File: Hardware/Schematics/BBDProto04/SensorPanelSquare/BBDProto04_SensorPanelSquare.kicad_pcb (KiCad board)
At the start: 2 copper layers, 223.5 x 238.8 mm, 94 parts, among them P1 CONN_02X08, P1-01 CONN_01X01, P1-02 CONN_01X01, P1-03 CONN_01X01, P1-04 CONN_01X01, P1-05 CONN_01X01, P1-06 CONN_01X01, P1-07 CONN_01X01, P1-08 CONN_01X01, P1-09 CONN_01X01, P1-10 CONN_01X01, P1-11 CONN_01X01, P1-12 CONN_01X01, P1-13 CONN_01X01, P1-14 CONN_01X01, P1-15 CONN_01X01, P1-16 CONN_01X01, P2 CONN_02X08, P2-01 CONN_01X01, P2-02 CONN_01X01, P2-03 CONN_01X01, P2-04 CONN_01X01, P2-05 CONN_01X01, P2-06 CONN_01X01, P2-07 CONN_01X01, P2-08 CONN_01X01, P2-09 CONN_01X01, P2-10 CONN_01X01, P2-11 CONN_01X01, P2-12 CONN_01X01, P2-13 CONN_01X01, P2-14 CONN_01X01, P2-15 CONN_01X01, P2-16 CONN_01X01, P3 CONN_02X08, P3-01 CONN_01X01, P3-02 CONN_01X01, P3-03 CONN_01X01, P3-04 CONN_01X01, P3-05 CONN_01X01, P3-06 CONN_01X01, P3-07 CONN_01X01, P3-08 CONN_01X01, P3-09 CONN_01X01, P3-10 CONN_01X01, P3-11 CONN_01X01, P3-12 CONN_01X01, P3-13 CONN_01X01, P3-14 CONN_01X01, P3-15 CONN_01X01, P3-16 CONN_01X01, P4 CONN_02X08, P4-01 CONN_01X01, P4-02 CONN_01X01, P4-03 CONN_01X01, P4-04 CONN_01X01, P4-05 CONN_01X01, P4-06 CONN_01X01, P4-07 CONN_01X01, P4-08 CONN_01X01, P4-09 CONN_01X01, P4-10 CONN_01X01, P4-11 CONN_01X01, P4-12 CONN_01X01, P4-13 CONN_01X01, P4-14 CONN_01X01, P4-15 CONN_01X01, P4-16 CONN_01X01

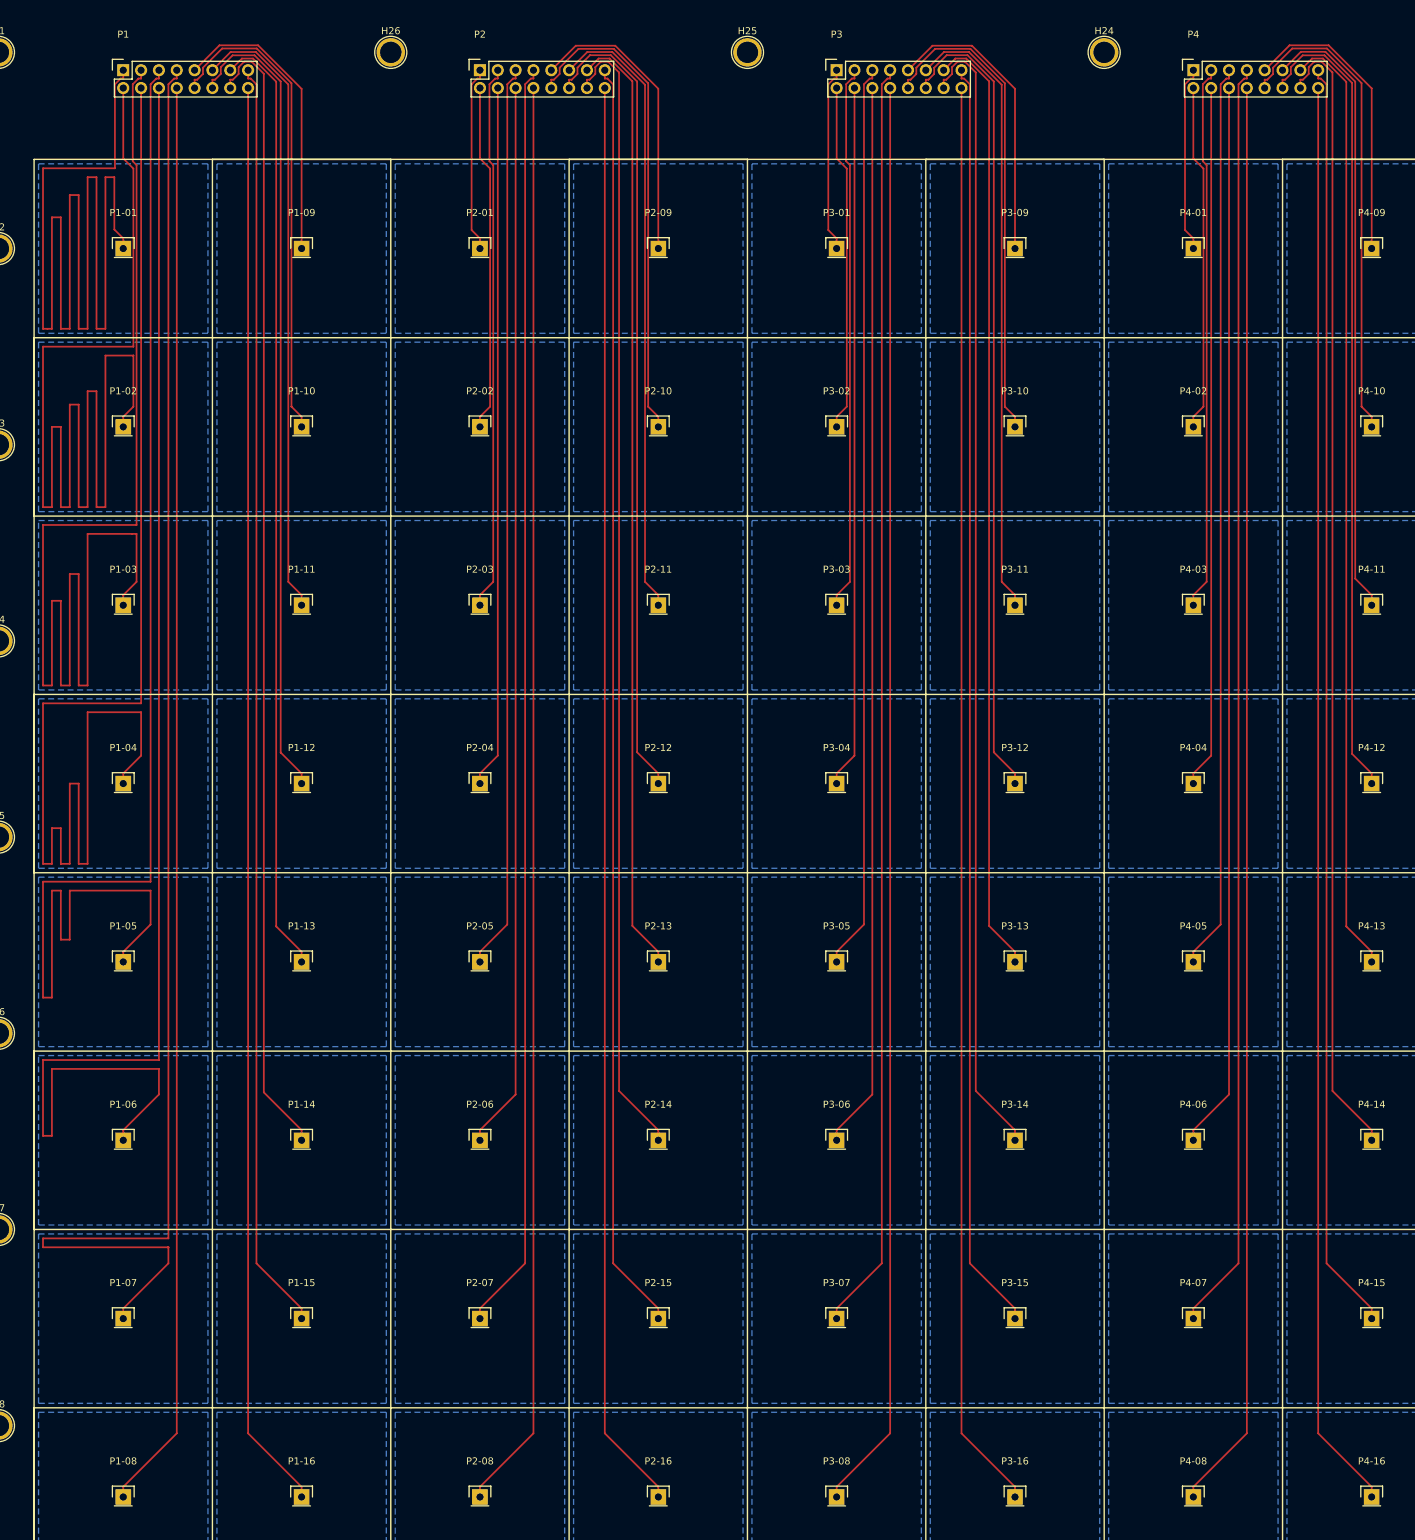
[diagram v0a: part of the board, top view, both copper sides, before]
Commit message: Proto #4 - Rev A
Proto #4 - Rev A
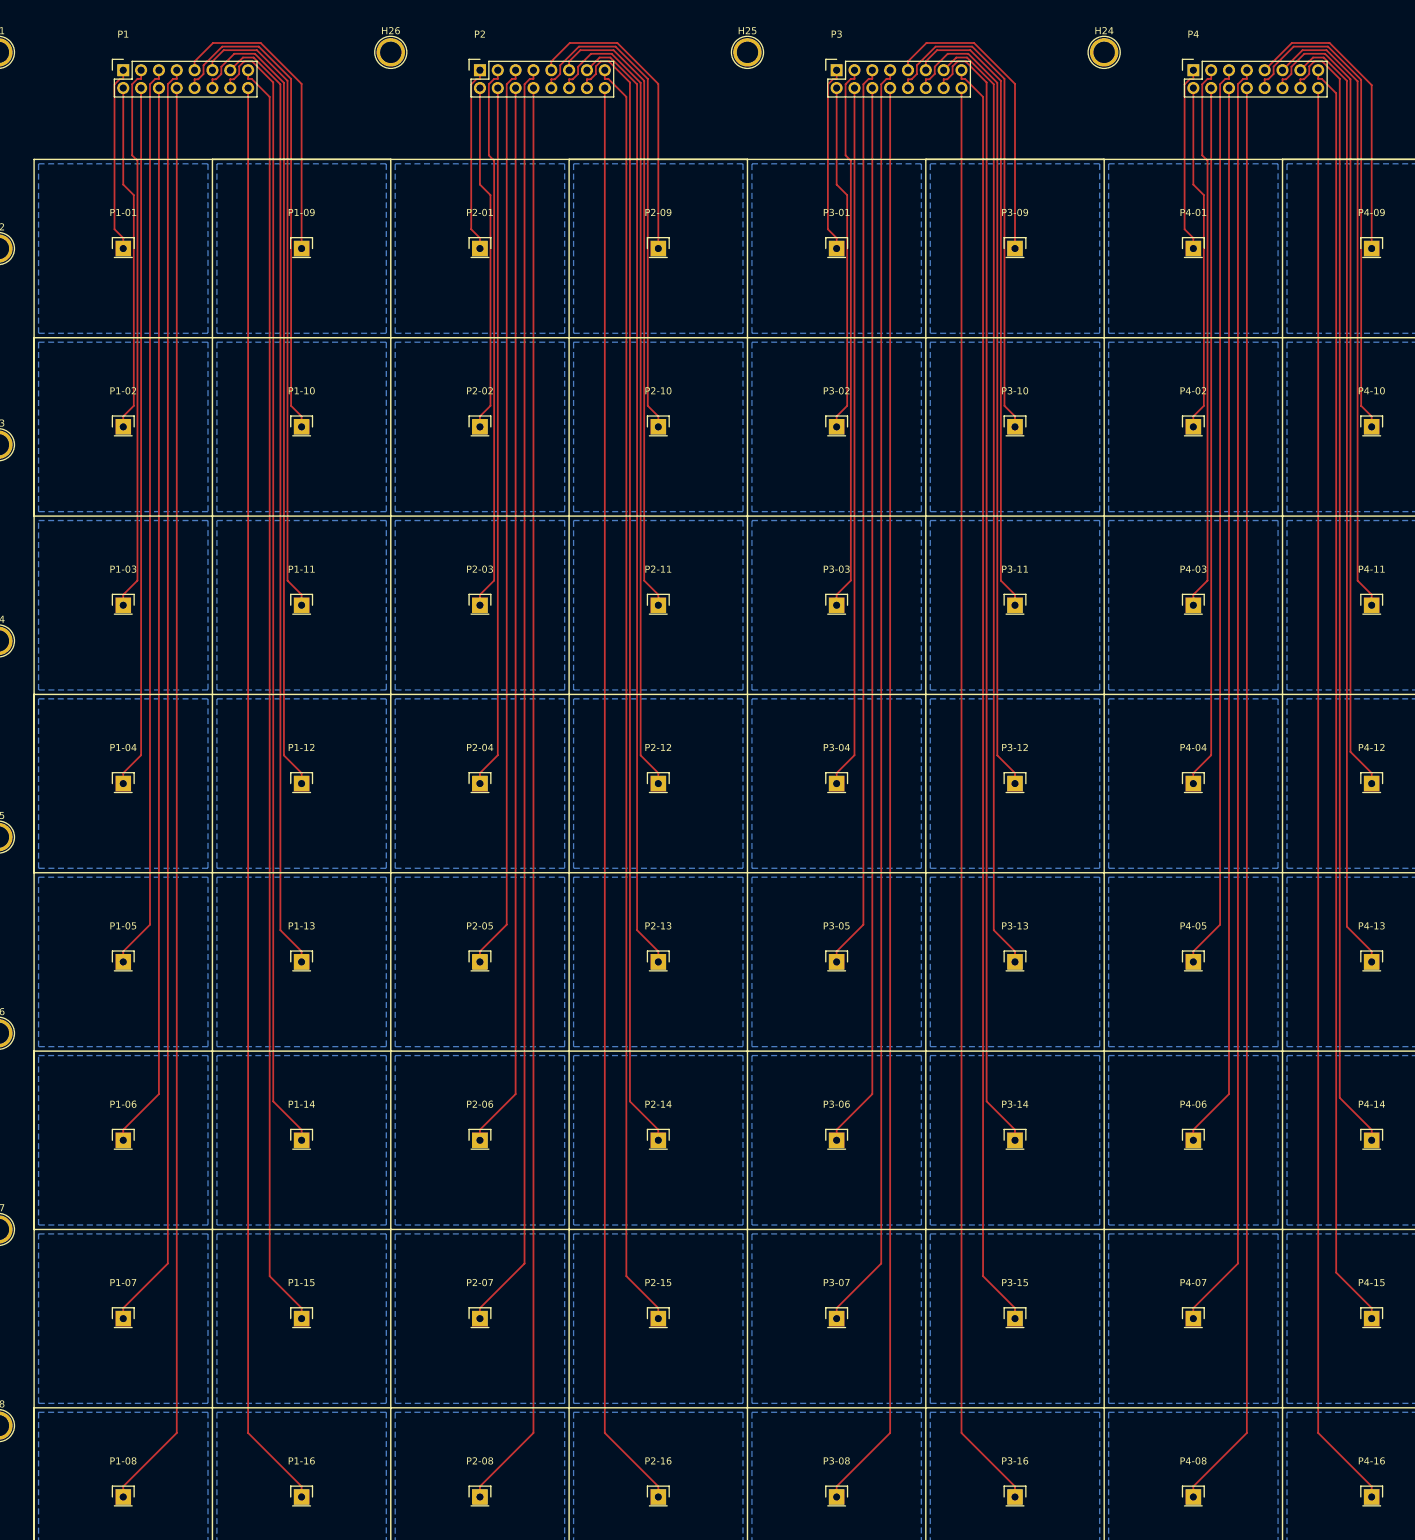
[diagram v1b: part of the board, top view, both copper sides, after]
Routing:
- net Net-(P1-01-Pad1): track 203.2 -> 26.7 mm
- net Net-(P1-02-Pad1): track 203.5 -> 49.5 mm
- net Net-(P1-03-Pad1): track 203.6 -> 78.2 mm
- net Net-(P1-04-Pad1): track 204.3 -> 100.1 mm
- net Net-(P1-05-Pad1): track 204.4 -> 129.4 mm
- net Net-(P1-06-Pad1): track 204.0 -> 152.0 mm
- net Net-(P1-07-Pad1): track 217.1 -> 181.3 mm
- net Net-(P3-09-Pad1): track 42.0 -> 43.4 mm
- net Net-(P2-09-Pad1): track 42.0 -> 43.4 mm
- net Net-(P1-09-Pad1): track 42.0 -> 43.4 mm
- net Net-(P3-11-Pad1): track 88.7 -> 89.9 mm
- net Net-(P2-11-Pad1): track 88.7 -> 89.9 mm
- net Net-(P1-11-Pad1): track 88.7 -> 89.9 mm
- net Net-(P3-10-Pad1): track 68.9 -> 69.7 mm
- net Net-(P2-10-Pad1): track 68.9 -> 69.7 mm
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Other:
- net class Default: clearance 0.2 -> 0.254; trace_width 0.25 -> 0.254
- rule trace_clearance: 0.2 -> 0.254
- board text added: "Bio Balance Detector #4 Rev. A (2016-05-02) | Square Sensor Panel | Andras Fuchs (andras.fuchs@gmail.com)"
- board text removed: "Bio Balance Detector Rev. B (2016-04-08) | Square Sensor Panel | Andras Fuchs (andras.fuchs@gmail.com)"
